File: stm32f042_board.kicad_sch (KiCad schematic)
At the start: 24 parts, among them J1 Conn_01x12_Female, J2 Conn_01x12_Female, J3 USB_B_Micro, J5 JTAG/SWD, U1 STM32F042F6Px, U2 MCP1802, U3 USBLC6-2SC6

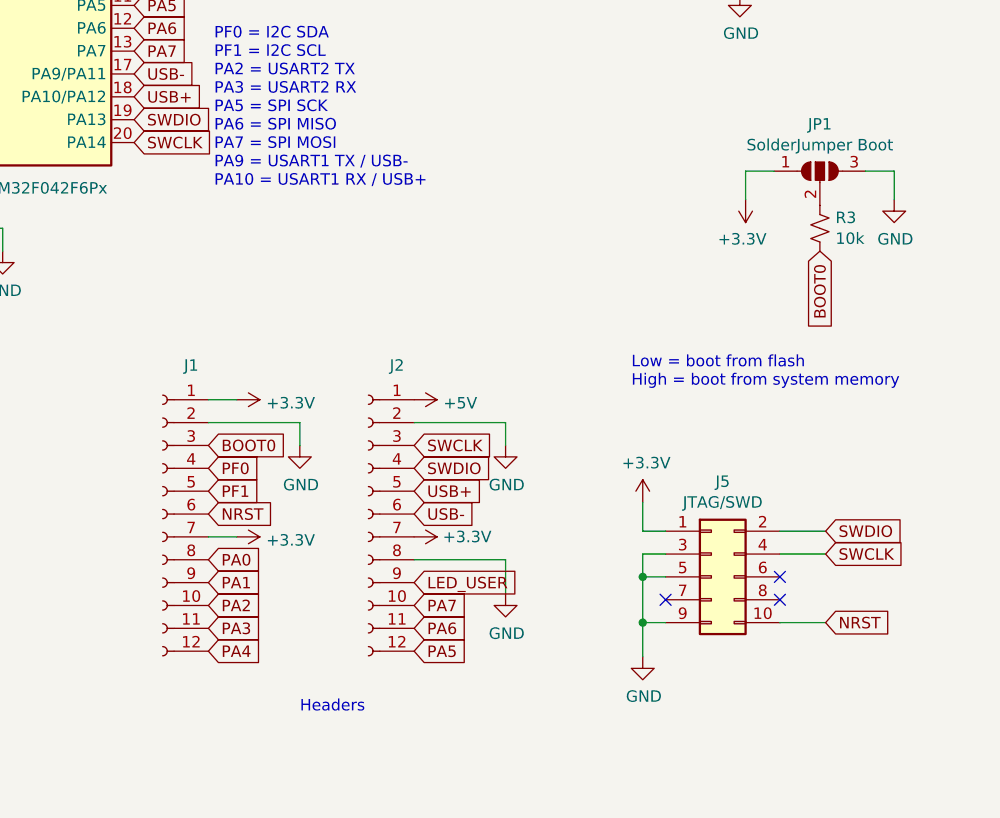
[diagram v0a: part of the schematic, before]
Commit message: Migrate to KiCad 7
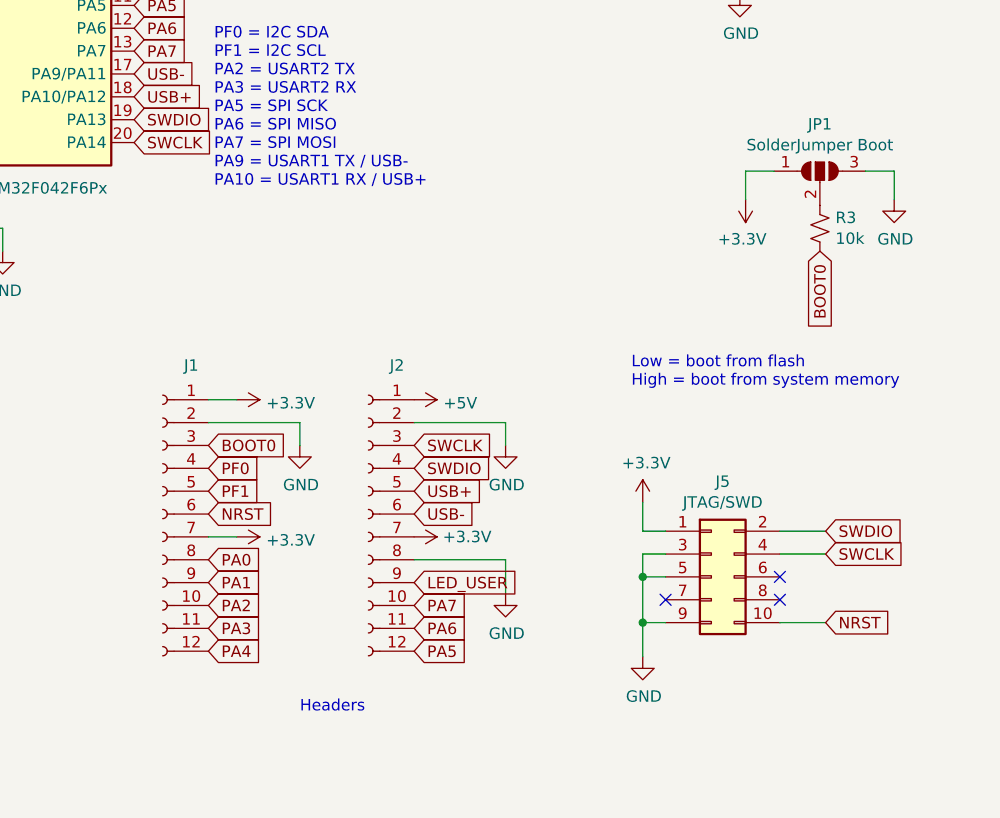
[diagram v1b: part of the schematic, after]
